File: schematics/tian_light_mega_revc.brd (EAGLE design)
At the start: 104.1 x 61.9 mm, 34 parts, among them IC2 MC33269ST-3.3T3, Q201 BUZ11

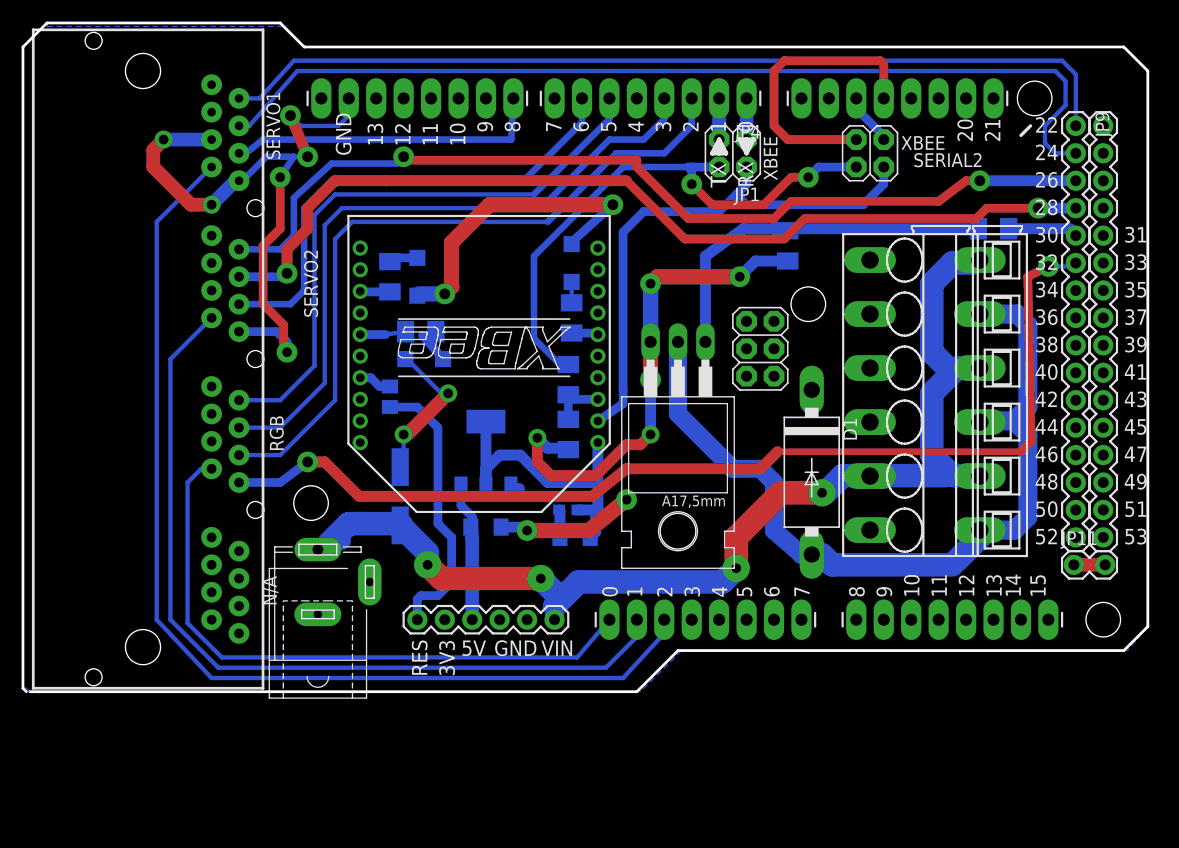
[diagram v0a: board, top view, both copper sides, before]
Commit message: -a
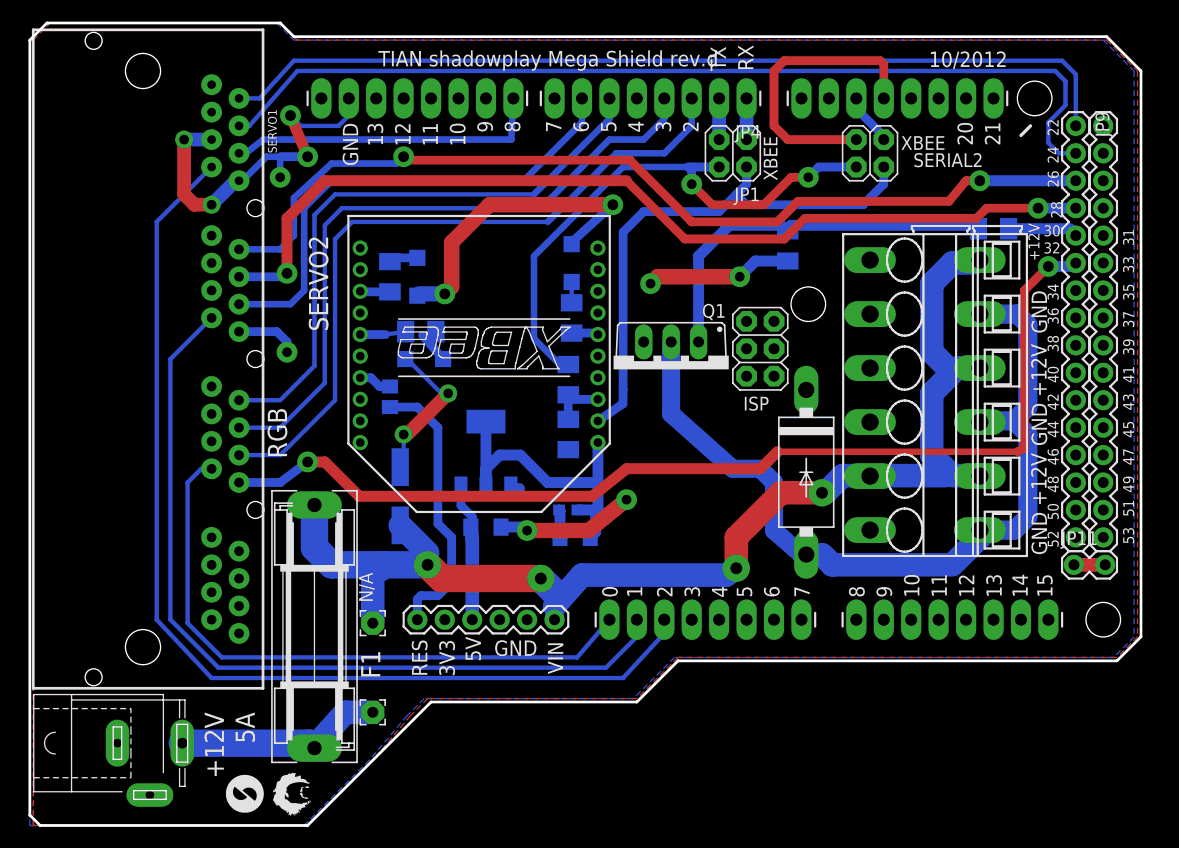
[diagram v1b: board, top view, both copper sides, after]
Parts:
- removed Q201: BUZ11, transistor-fet:TO220
- added F1: (no value), fuse:SH22,5
- added PAD1, PAD2: (no value), wirepad:2,15/1,0
- added Q1: IRF530, transistor-power:TO220BV
- moved J201 21.6 mm to (-2.54, -8.26), turned to 0 degrees
- moved D1 0.51 mm to (58.2, 16.8)
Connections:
- new net N$10: F1.1, J201.3, PAD1.1
- net 12V: now also F1.2, PAD2.1; no longer J201.3
- net DRAIN: now also Q1.D; no longer Q201.2
- net GND: now also Q1.S; no longer Q201.3
- net N$3: now also Q1.G; no longer Q201.1
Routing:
- net GND: track 171.1 -> 117.3 mm, vias 17 -> 14
- net N$10: track 0.00 -> 19.2 mm
- net 12V: track 110.5 -> 118.9 mm
- net D32: track 97.3 -> 96.7 mm
- net D28: track 87.1 -> 87.7 mm
- added copper zone on layer 1, net GND
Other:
- board size 104.1 x 61.9 mm -> 102.9 x 74.3 mm
- board text added: "+12V"
- board text added: "10/2012"
- board text added: "5A"
- board text added: "ISP"
- board text added: "TIAN shadowplay Mega Shield rev.d"
